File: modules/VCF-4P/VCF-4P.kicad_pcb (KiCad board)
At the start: 2 copper layers, 111.3 x 108.2 mm, 68 parts, among them J1 WQP-PJ398, J10 Conn_Front_Left, J11 Conn_Back_Right, J12 Conn_Front_Right, J13 Conn_Back_Left, J3 WQP-PJ398, J5 WQP-PJ398, J7 WQP-PJ398, J8 WQP-PJ398, J9 Conn_Eurorack_16, U1 SSI2140, U2 TL074

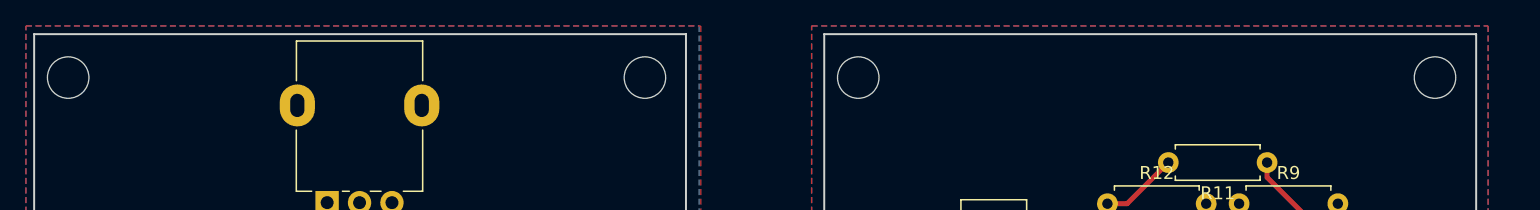
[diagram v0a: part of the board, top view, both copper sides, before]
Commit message: VCF-4P: PCB layout - wip
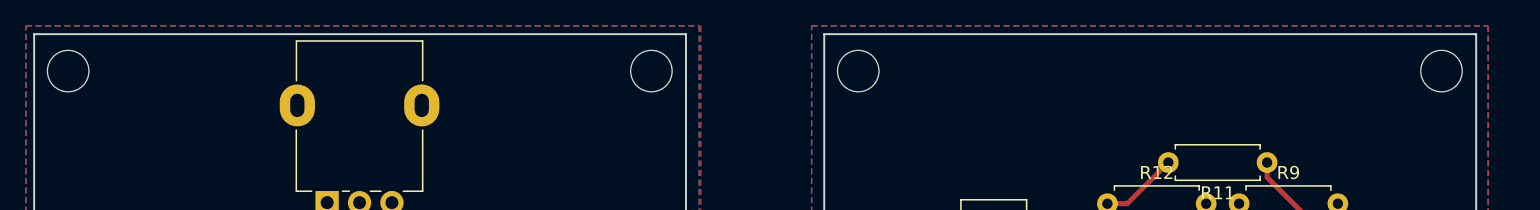
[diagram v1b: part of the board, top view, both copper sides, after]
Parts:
- moved H2 0.71 mm to (144.1, 38.4)
- moved H6 0.71 mm to (205.1, 38.4)
- moved H1 0.50 mm to (99.1, 38.4)
- moved H3 0.50 mm to (160.1, 38.4)
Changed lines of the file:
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@@
   )
   (footprint "-lmp-holes:MountingHole_PCB_3.2mm_M3" locked (layer "F.Cu")
-    (at 204.605 38.91)
+    (at 205.105 38.41)
     (descr "Mounting Hole 3.2mm, no annular, M3")
     (tags "mounting hole 3.2mm m3")
@@
   )
   (footprint "-lmp-holes:MountingHole_PCB_3.2mm_M3" locked (layer "F.Cu")
-    (at 99.145 38.91)
+    (at 99.145 38.41)
     (descr "Mounting Hole 3.2mm, no annular, M3")
     (tags "mounting hole 3.2mm m3")
@@
   )
   (footprint "-lmp-holes:MountingHole_PCB_3.2mm_M3" locked (layer "F.Cu")
-    (at 143.645 38.91)
+    (at 144.145 38.41)
     (descr "Mounting Hole 3.2mm, no annular, M3")
     (tags "mounting hole 3.2mm m3")
@@
   )
   (footprint "-lmp-holes:MountingHole_PCB_3.2mm_M3" locked (layer "F.Cu")
-    (at 160.105 38.91)
+    (at 160.105 38.41)
     (descr "Mounting Hole 3.2mm, no annular, M3")
     (tags "mounting hole 3.2mm m3")

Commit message: VCF-4P: PCB layout - wip
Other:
- board text added: "TODO: Adjust control positions"
- board text removed: "TODO: Adjust control & connector positions"
- board text removed: "TODO: Verify headers match control PCB"
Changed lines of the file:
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@@
   )
   (gr_line (start 192.4304 142.621) (end 189.357 142.621) (layer "F.SilkS") (width 0.3048))
-  (gr_line (start 142.621 56.91) (end 149.733 56.91) (layer "Dwgs.User") (width 0.1016))
-  (gr_line (start 206.06 53.707) (end 206.06 58.406) (layer "Dwgs.User") (width 0.1016))
-  (gr_line (start 203.581 56.91) (end 210.693 56.91) (layer "Dwgs.User") (width 0.1016))
-  (gr_line (start 98.3 54.5605) (end 98.3 59.2595) (layer "Dwgs.User") (width 0.1016))
-  (gr_line (start 156.652 56.91) (end 163.764 56.91) (layer "Dwgs.User") (width 0.1016))
-  (gr_line (start 94.742 56.91) (end 101.854 56.91) (layer "Dwgs.User") (width 0.1016))
-  (gr_line (start 145.1 53.864) (end 145.1 58.563) (layer "Dwgs.User") (width 0.1016))
-  (gr_line (start 159.26 53.721) (end 159.26 58.42) (layer "Dwgs.User") (width 0.1016))
   (gr_line (start 157.48 143.764) (end 157.48 35.56) (layer "Edge.Cuts") (width 0.1524))
   (gr_line (start 157.48 35.56) (end 207.78 35.56) (layer "Edge.Cuts") (width 0.1524))
@@
     (effects (font (size 1 1) (thickness 0.15)) (justify left))
   )
-  (gr_text "TODO: Adjust control & connector positions" (at 121.666 52.451) (layer "Cmts.User")
+  (gr_text "TODO: Adjust control positions" (at 121.666 52.451) (layer "Cmts.User")
     (effects (font (size 1.016 1.016) (thickness 0.1524)))
   )
@@
     (effects (font (size 1.016 1.016) (thickness 0.1524)))
   )
-  (gr_text "TODO: Verify headers \nmatch control PCB" (at 210.693 108.204 90) (layer "Cmts.User")
-    (effects (font (size 1.016 1.016) (thickness 0.1524)))
-  )
